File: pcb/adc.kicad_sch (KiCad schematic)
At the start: 4 parts, among them U7 ADS1220

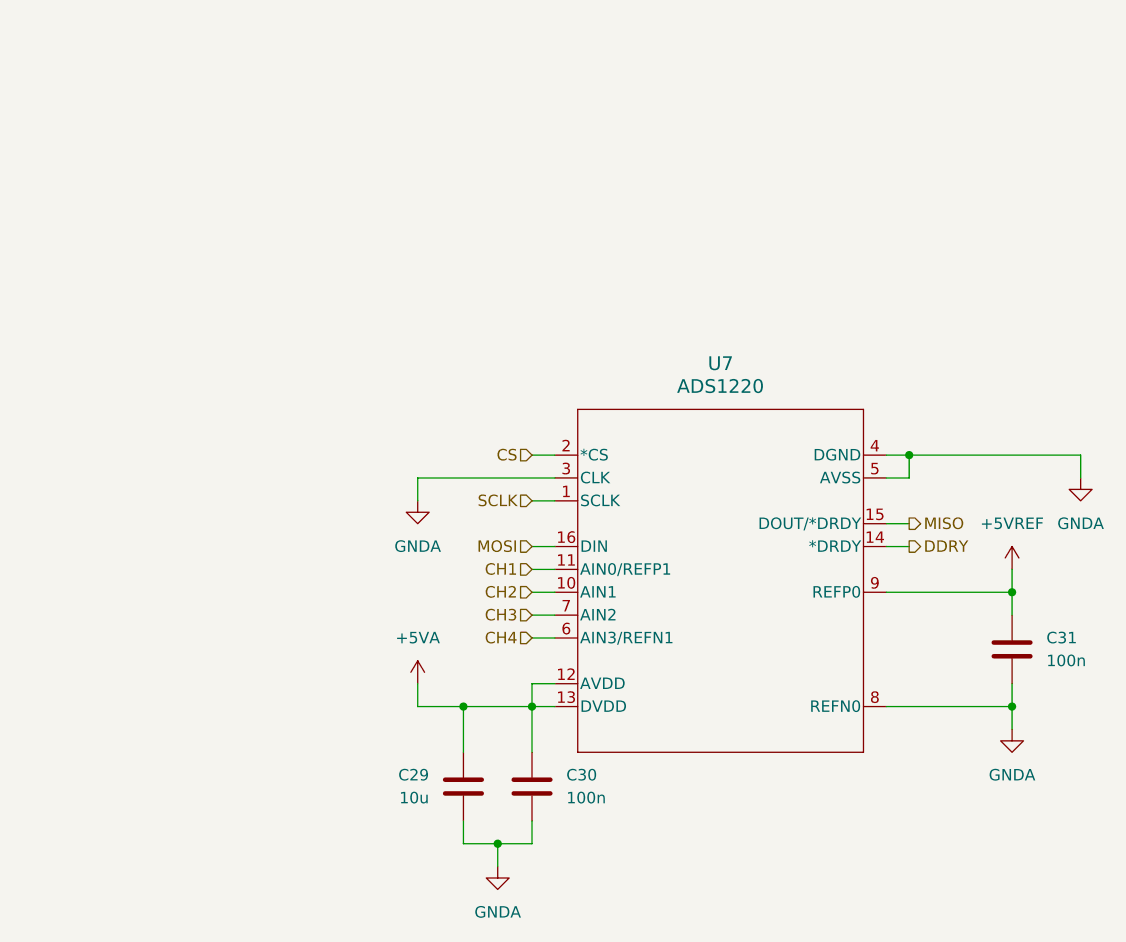
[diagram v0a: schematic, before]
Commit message: chore: many changes checkpoint
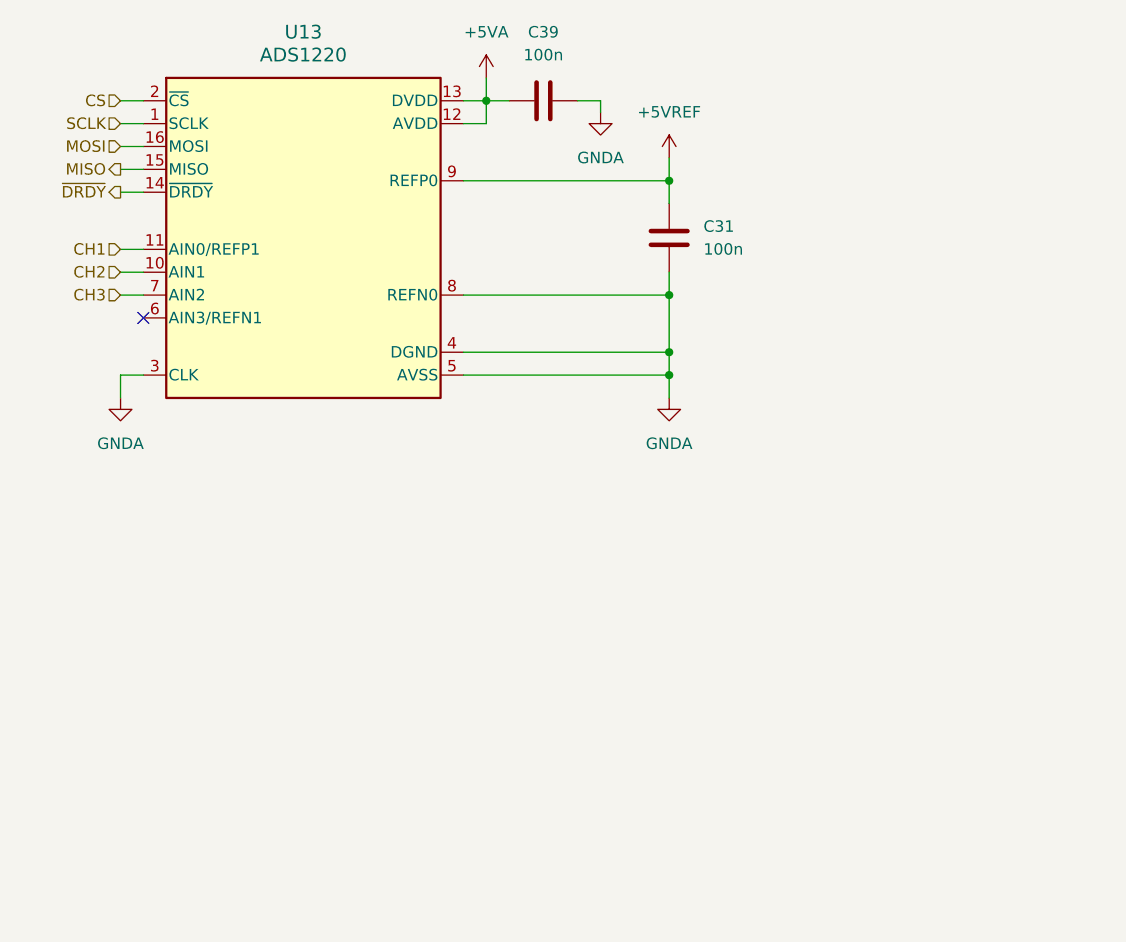
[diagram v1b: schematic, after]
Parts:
- removed C29: 10u, symbol Device:C
- removed C30: 100n, symbol Device:C
- removed U7: ADS1220, PW16, symbol project_library:ADS1220
- added C39: 100n, Capacitor_SMD:C_0603_1608Metric, symbol Device:C
- added U13: ADS1220, Package_SO:TSSOP-16_4.4x5mm_P0.65mm, symbol project_library:ADS1220
- C31: footprint (none) -> Capacitor_SMD:C_0603_1608Metric
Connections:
- net +5VA: now also C39.1, U13.12 (AVDD), U13.13 (DVDD)
- net +5VREF: now also U13.9 (REFP0)
- net CH1: now also U13.11 (AIN0/REFP1)
- net CH2: now also U13.10 (AIN1)
- net CH3: now also U13.7 (AIN2)
- net CS: now also U13.2 (~{CS})
- net GNDA: now also C39.2, U13.3 (CLK), U13.4 (DGND), U13.5 (AVSS), U13.8 (REFN0)
- net MISO: now also U13.15 (MISO)
- net MOSI: now also U13.16 (MOSI)
- net SCLK: now also U13.1 (SCLK)
- new net ~{DRDY}: U13.14 (~{DRDY})
- no-connect marks 0 -> 1
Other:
- moved on the sheet: C31
